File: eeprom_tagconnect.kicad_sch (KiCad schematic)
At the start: 7 parts, among them J1 Tag-Connect_TC2050-IDC-NL_2x5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, U5 25LC512, U7 NVT4858_XQFN

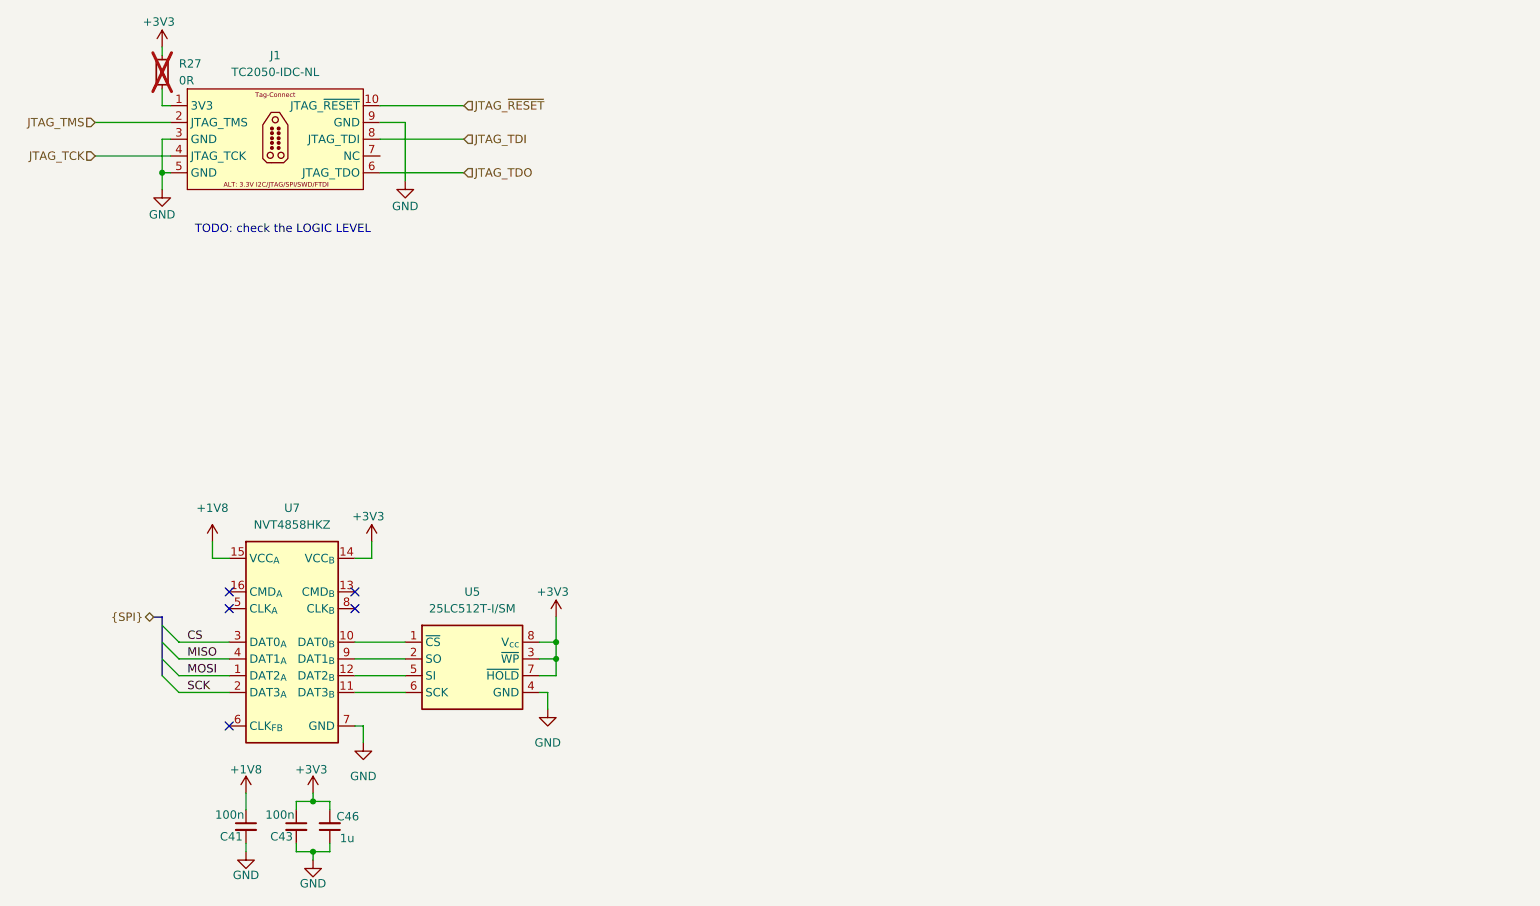
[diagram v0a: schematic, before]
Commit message: [#100765] Update schematic
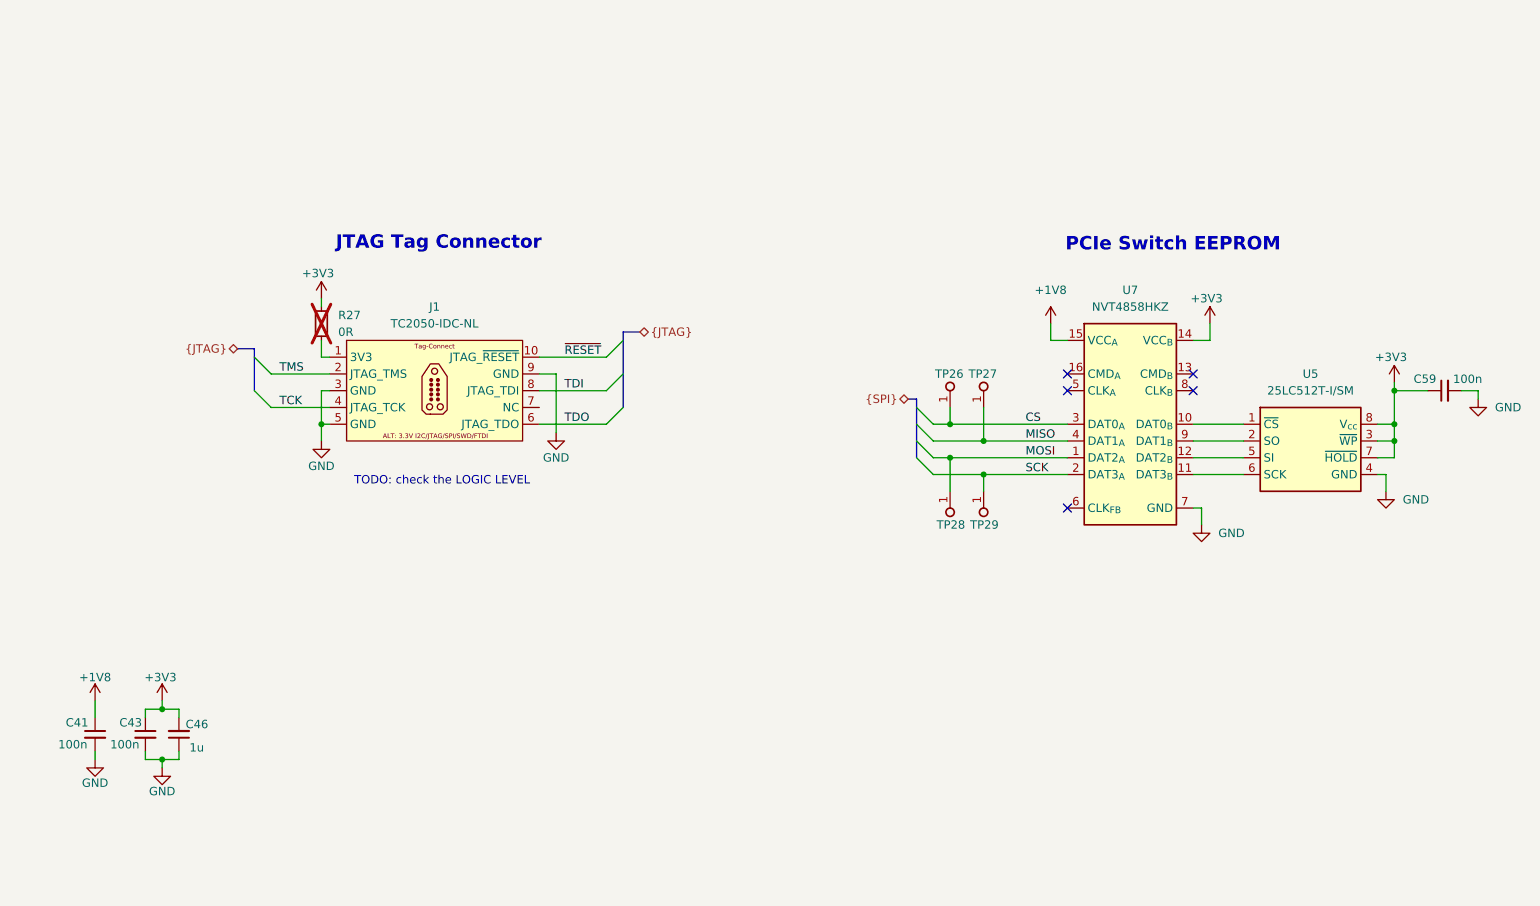
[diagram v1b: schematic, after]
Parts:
- added C59: C_100n_0402, antmicro-footprints:C_0402_1005Metric, symbol antmicroCapacitors0402:C_100n_0402
- added TP26, TP27, TP28, TP29: TP_0.75mm_SMD, antmicro-footprints:TP_SMD_0.75mm, symbol antmicroTestPoints:TP_0.75mm_SMD
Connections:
- net +3V3: now also C59.1
- net CS: now also TP26.1
- net GND: now also C59.2
- net MISO: now also TP27.1
- net MOSI: now also TP28.1
- net SCK: now also TP29.1
- net JTAG_TCK renamed TCK
- net JTAG_TDI renamed TDI
- net JTAG_TDO renamed TDO
- net JTAG_TMS renamed TMS
- net JTAG_~{RESET} renamed ~{RESET}
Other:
- note added: "JTAG Tag Connector"
- note added: "PCIe Switch EEPROM"
- moved on the sheet: C41, C43, C46, J1, R27, U5, U7

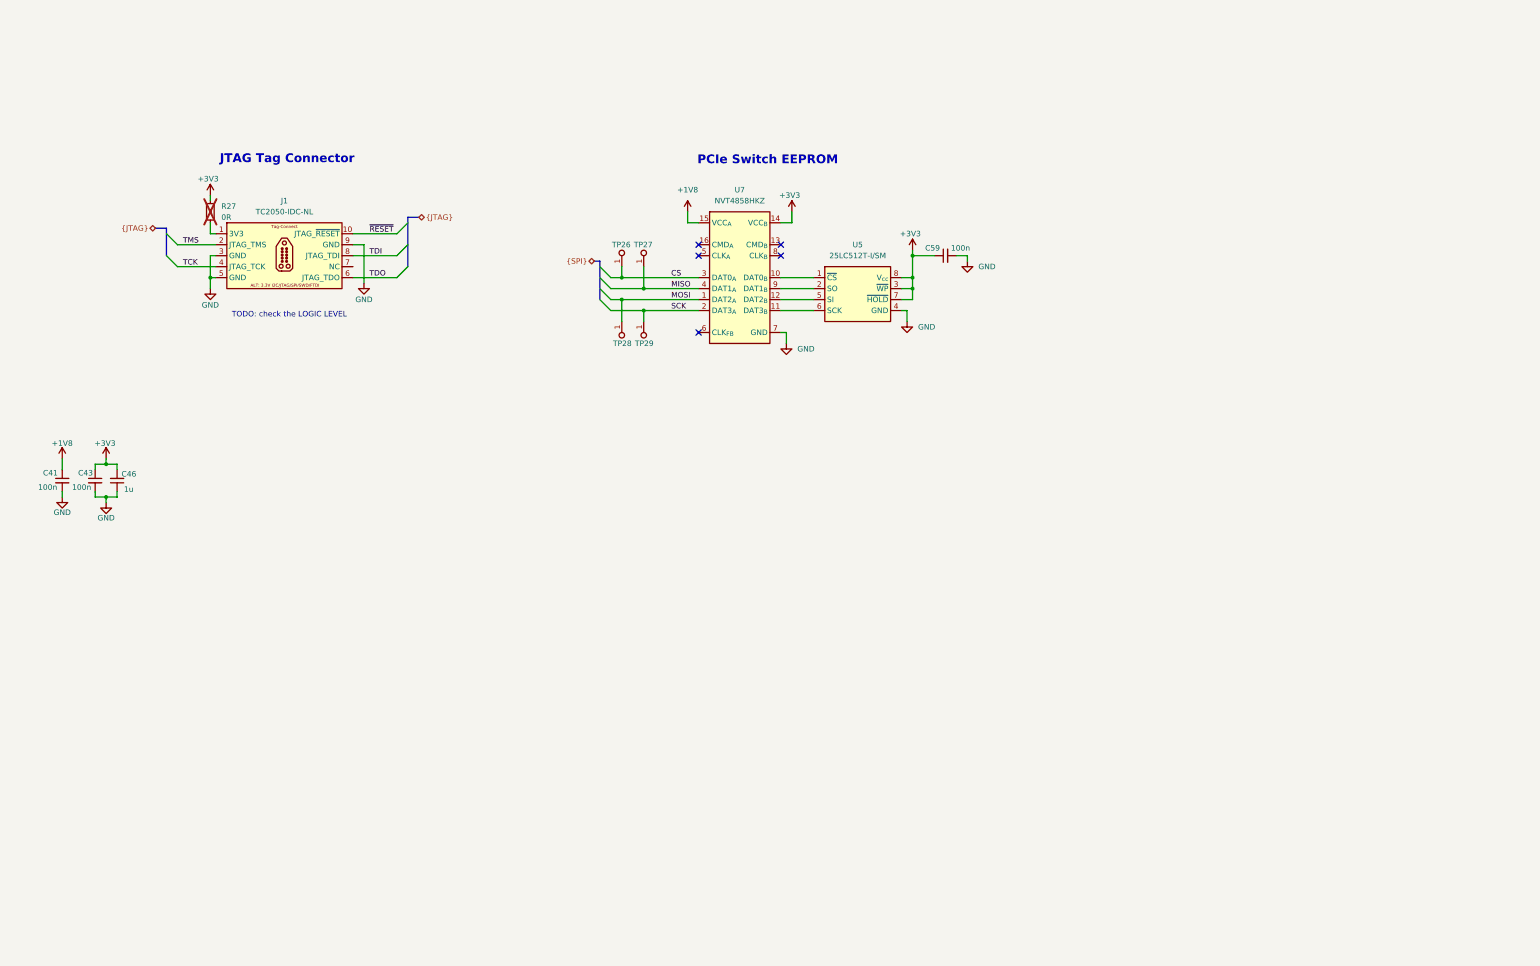
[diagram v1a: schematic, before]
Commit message: [#100765] Change LLC
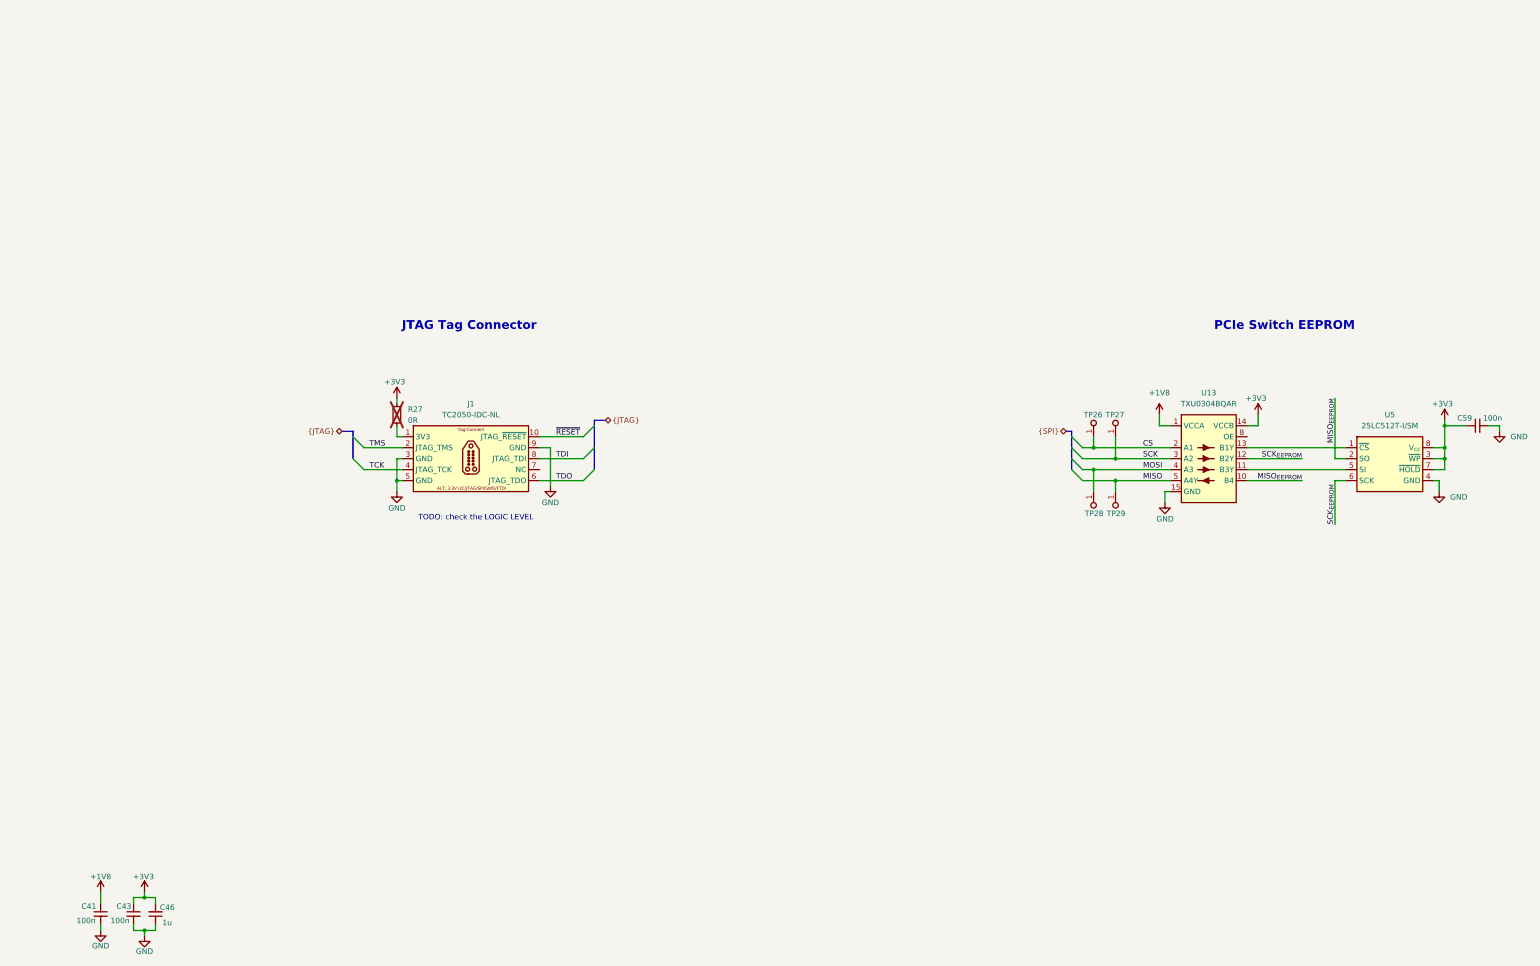
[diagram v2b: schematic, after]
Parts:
- removed U7: NVT4858_XQFN, antmicro-footprints:SOT1161-2, symbol antmicroLogicTranslatorsLevelShifters:NVT4858_XQFN
- added U13: TXU0304BQAR, antmicro-footprints:DHVQFN-14-1EP_2.5x3mm, symbol antmicroLogicTranslatorsLevelShifters:TXU0304BQAR
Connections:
- net +1V8: now also U13.1 (VCCA)
- net +3V3: now also U13.14 (VCCB)
- net CS: now also U13.2 (A1)
- net GND: now also U13.15 (GND), U13.7 (GND)
- net MISO: now also TP29.1, U13.5 (A4Y); no longer TP27.1
- net MOSI: now also U13.4 (A3)
- net SCK: now also TP27.1, U13.3 (A2); no longer TP29.1
- net at U5.1 (~{CS}): now also U13.13 (B1Y)
- net SCK_{EEPROM}: now reaches U5.6 (SCK)
- net SCK_{EEPROM}: now also U13.12 (B2Y)
- net at U5.5 (SI): now also U13.11 (B3Y)
- net MISO_{EEPROM}: now reaches U5.2 (SO)
- net MISO_{EEPROM}: now also U13.10 (B4)
- no-connect marks 5 -> 0
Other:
- company: (none) -> Antmicro
- title: (none) -> antmicro-jetson-orin-baseboard-pcie-switch-expansion-hw
- moved on the sheet: C41, C43, C46, C59, J1, R27, TP26, TP27, TP28, TP29, U5
